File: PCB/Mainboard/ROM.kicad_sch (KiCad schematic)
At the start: 16 parts, among them Q35 8C, Q36 7C, U24 E4, U60 E3

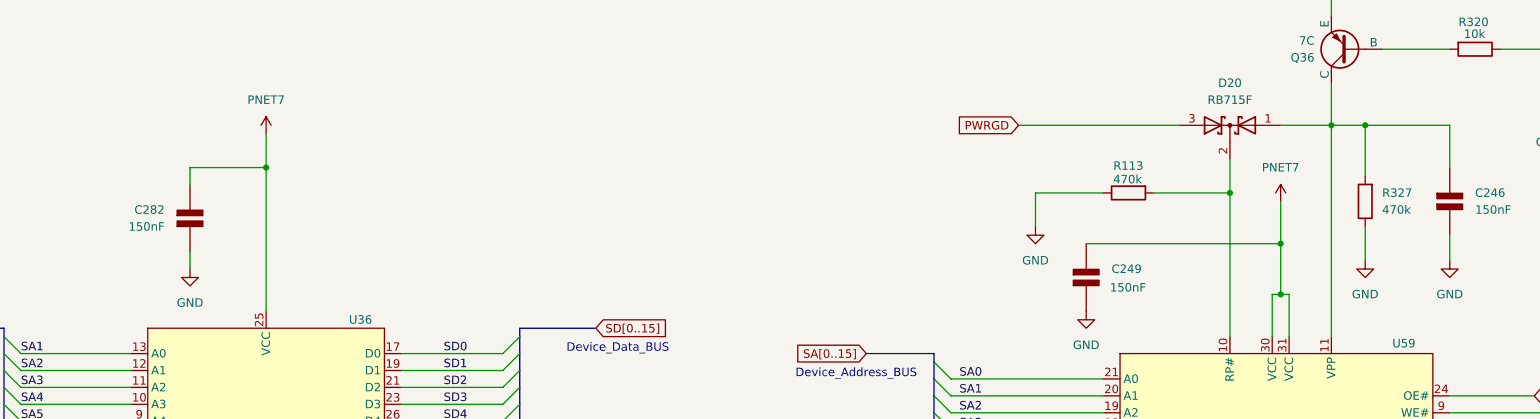
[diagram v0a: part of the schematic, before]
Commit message: Add files via upload
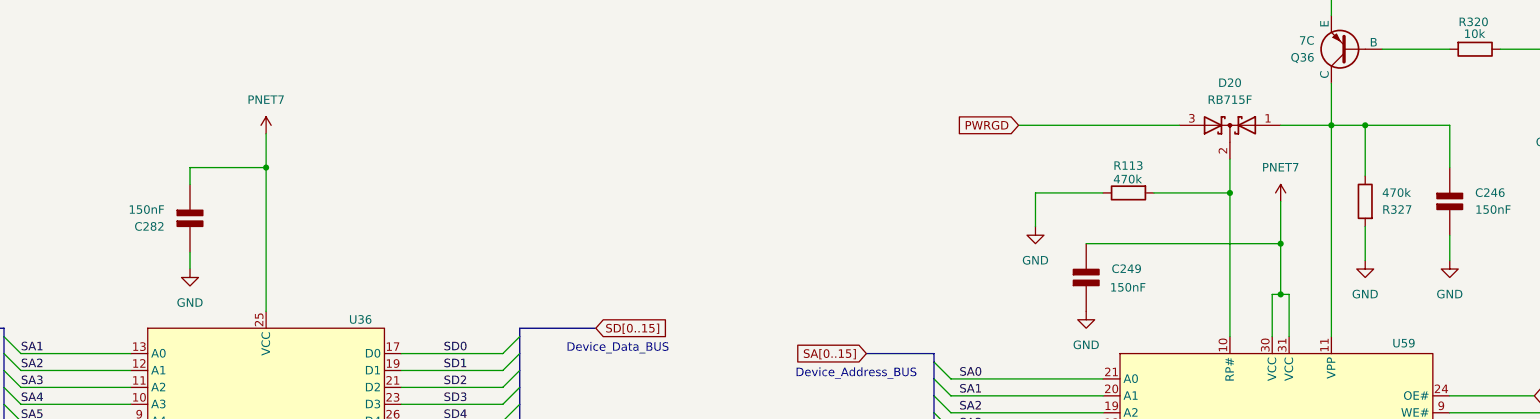
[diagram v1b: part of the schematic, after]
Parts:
- C246: footprint (none) -> Capacitor_SMD:C_0603_1608Metric
- C249, C282: footprint (none) -> Capacitor_SMD:C_0402_1005Metric
- D19, D20: footprint (none) -> PC110:SOT-416L
- Q35: footprint Package_TO_SOT_SMD:SOT-23 -> Package_TO_SOT_SMD:SOT-523
- Q36: footprint (none) -> Package_TO_SOT_SMD:TSOT-23
- R112, R113, R320, R321, R327: footprint (none) -> PCM_Resistor_SMD_AKL:R_0402_1005Metric
- U24, U60: footprint (none) -> PC110:SOT-353
- U36: footprint (none) -> PC110:SOP48
- U59: footprint (none) -> PC110:Flash-40
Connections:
- net GND: now also C282.2 (-), R327.2; no longer C282.1 (+), R327.1
- net PNET7: now also C282.1 (+); no longer C282.2 (-)
- net at C246.1 (+), D20.1 (A), Q36.1 (C)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: now also R327.1; no longer R327.2
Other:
- moved on the sheet: R327
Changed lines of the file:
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@@
 			)
 		)
-		(property "Footprint" ""
+		(property "Footprint" "PCM_Resistor_SMD_AKL:R_0402_1005Metric"
 			(at 314.96 101.092 90)
 			(effects
@@
 			)
 		)
-		(property "Footprint" ""
+		(property "Footprint" "PC110:Flash-40"
 			(at 252.73 157.48 0)
 			(effects
@@
 			)
 		)
-		(property "Footprint" ""
+		(property "Footprint" "PC110:SOT-416L"
 			(at 245.11 99.06 0)
 			(effects
@@
 			)
 		)
-		(property "Footprint" ""
+		(property "Footprint" "PC110:SOT-353"
 			(at 337.82 102.87 0)
 			(effects
@@
 			)
 		)
-		(property "Footprint" ""
+		(property "Footprint" "Package_TO_SOT_SMD:TSOT-23"
 			(at 227.33 87.63 0)
 			(effects
@@
 		(lib_id "PCM_Elektuur:C")
 		(at 88.9 113.03 0)
-		(mirror x)
 		(unit 1)
 		(exclude_from_sim no)
@@
 		(dnp no)
 		(property "Reference" "C282"
-			(at 85.09 111.7599 0)
+			(at 85.09 114.3001 0)
 			(effects
 				(font
@@
 		)
 		(property "Value" "150nF"
-			(at 85.09 114.2999 0)
+			(at 85.09 111.7601 0)
 			(effects
 				(font
@@
 			)
 		)
-		(property "Footprint" ""
+		(property "Footprint" "Capacitor_SMD:C_0402_1005Metric"
 			(at 88.9 113.03 0)
 			(effects
@@
 		)
 		(property "Indicator" "+"
-			(at 87.63 116.205 0)
+			(at 87.63 109.855 0)
 			(effects
 				(font
@@
 		)
 		(property "Rating" "V"
-			(at 88.265 109.855 0)
+			(at 88.265 116.205 0)
 			(effects
 				(font
@@
 			)
 		)
-		(property "Footprint" ""
+		(property "Footprint" "PCM_Resistor_SMD_AKL:R_0402_1005Metric"
 			(at 229.87 107.442 90)
 			(effects
@@
 			)
 		)
-		(property "Footprint" ""
+		(property "Footprint" "PCM_Resistor_SMD_AKL:R_0402_1005Metric"
 			(at 281.94 85.852 90)
 			(effects
@@
 			)
 		)
-		(property "Footprint" ""
+		(property "Footprint" "PC110:SOP48"
 			(at 100.33 158.75 0)
 			(effects
@@
 			)
 		)
-		(property "Footprint" ""
+		(property "Footprint" "Capacitor_SMD:C_0603_1608Metric"
 			(at 278.13 110.49 0)
 			(effects
@@
 			)
 		)
-		(property "Footprint" "Package_TO_SOT_SMD:SOT-23"
+		(property "Footprint" "Package_TO_SOT_SMD:SOT-523"
 			(at 294.64 104.775 0)
 			(effects
@@
 			)
 		)
-		(property "Footprint" ""
+		(property "Footprint" "Capacitor_SMD:C_0402_1005Metric"
 			(at 223.52 121.92 0)
 			(effects
@@
 			)
 		)
-		(property "Footprint" ""
+		(property "Footprint" "PC110:SOT-416L"
 			(at 375.92 195.58 0)
 			(effects
@@
 	(symbol
 		(lib_id "Device:R")
-		(at 265.43 110.49 180)
-		(unit 1)
-		(exclude_from_sim no)
-		(in_bom yes)
-		(on_board yes)
-		(dnp no)
-		(fields_autoplaced yes)
+		(at 265.43 110.49 0)
+		(mirror y)
+		(unit 1)
+		(exclude_from_sim no)
+		(in_bom yes)
+		(on_board yes)
+		(dnp no)
 		(property "Reference" "R327"
-			(at 267.97 109.2199 0)
+			(at 267.97 111.7601 0)
 			(effects
 				(font
@@
 		)
 		(property "Value" "470k"
-			(at 267.97 111.7599 0)
+			(at 267.97 109.2201 0)
 			(effects
 				(font
@@
 			)
 		)
-		(property "Footprint" ""
+		(property "Footprint" "PCM_Resistor_SMD_AKL:R_0402_1005Metric"
 			(at 267.208 110.49 90)
 			(effects
@@
 			)
 		)
-		(property "Footprint" ""
+		(property "Footprint" "PCM_Resistor_SMD_AKL:R_0402_1005Metric"
 			(at 374.142 168.91 90)
 			(effects
@@
 			)
 		)
-		(property "Footprint" ""
+		(property "Footprint" "PC110:SOT-353"
 			(at 337.82 142.24 0)
 			(effects

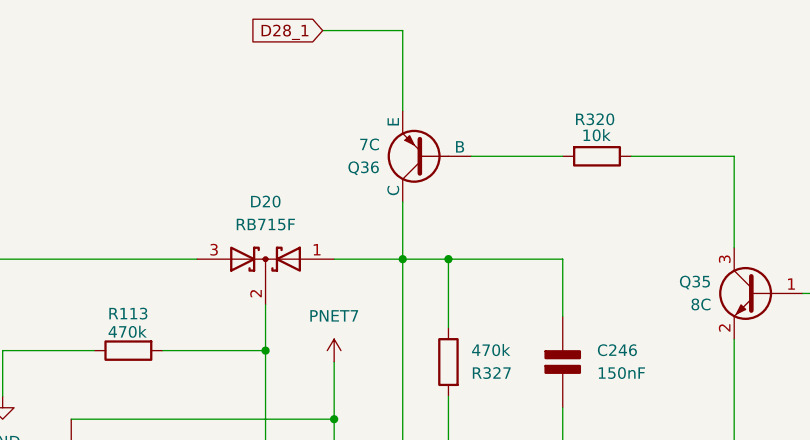
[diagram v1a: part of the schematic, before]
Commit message: Add files via upload
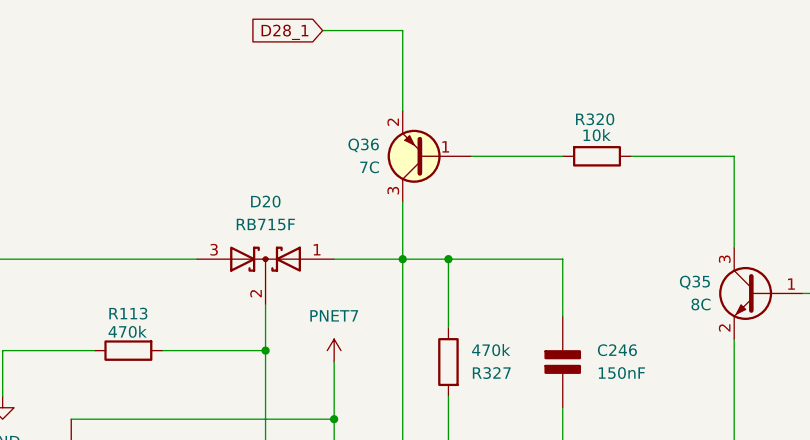
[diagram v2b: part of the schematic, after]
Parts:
- removed Q36: 7C, Package_TO_SOT_SMD:TSOT-23, symbol Simulation_SPICE:PNP
- added Q36: 7C, symbol PCM_Transistor_BJT_AKL:Q_PNP_Generic_BEC
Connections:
- net D28_1: now also Q36.2 (E)
- net at C246.1 (+), D20.1 (A), R327.1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: now also Q36.3 (C)
- net at R320.2: now also Q36.1 (B)
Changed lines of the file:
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@@
 	)
 	(symbol
-		(lib_id "Simulation_SPICE:PNP")
-		(at 262.89 87.63 180)
+		(lib_id "PCM_Transistor_BJT_AKL:Q_PNP_Generic_BEC")
+		(at 262.89 87.63 0)
+		(mirror y)
 		(unit 1)
 		(exclude_from_sim no)
@@
 		(dnp no)
 		(property "Reference" "Q36"
-			(at 257.81 88.9001 0)
+			(at 257.81 86.3599 0)
 			(effects
 				(font
@@
 		)
 		(property "Value" "7C"
-			(at 257.81 86.3601 0)
+			(at 257.81 88.8999 0)
 			(effects
 				(font
@@
 			)
 		)
-		(property "Footprint" "Package_TO_SOT_SMD:TSOT-23"
-			(at 227.33 87.63 0)
+		(property "Footprint" ""
+			(at 257.81 90.17 0)
 			(effects
 				(font
@@
 			)
 		)
-		(property "Datasheet" "https://ngspice.sourceforge.io/docs/ngspice-html-manual/manual.xhtml#cha_BJTs"
-			(at 227.33 87.63 0)
-			(effects
-				(font
-					(size 1.27 1.27)
-				)
-				(hide yes)
-			)
-		)
-		(property "Description" "Bipolar transistor symbol for simulation only, substrate tied to the emitter"
+		(property "Datasheet" "~"
 			(at 262.89 87.63 0)
 			(effects
@@
 			)
 		)
-		(property "Sim.Device" "PNP"
+		(property "Description" "PNP transistor, generic symbol, Alternate KiCAD Library"
 			(at 262.89 87.63 0)
 			(effects
@@
 			)
 		)
-		(property "Sim.Type" "GUMMELPOON"
-			(at 262.89 87.63 0)
-			(effects
-				(font
-					(size 1.27 1.27)
-				)
-				(hide yes)
-			)
-		)
-		(property "Sim.Pins" "1=C 2=B 3=E"
-			(at 262.89 87.63 0)
-			(effects
-				(font
-					(size 1.27 1.27)
-				)
-				(hide yes)
-			)
-		)
-		(pin "3"
-		)
 		(pin "1"
 		)
 		(pin "2"
 		)
+		(pin "3"
+		)
 		(instances
-			(project ""
+			(project "PC110"
 				(path "/45c7911f-b027-440e-9e3e-77a146b41944/29aeee43-2869-4080-920c-a693b0bc5770"
 					(reference "Q36")
